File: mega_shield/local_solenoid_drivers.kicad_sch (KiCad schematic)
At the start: 15 parts, among them J21 1803277, J7 1803277, Q43 AO4486, Q44 AO4486, U29 NUP2202

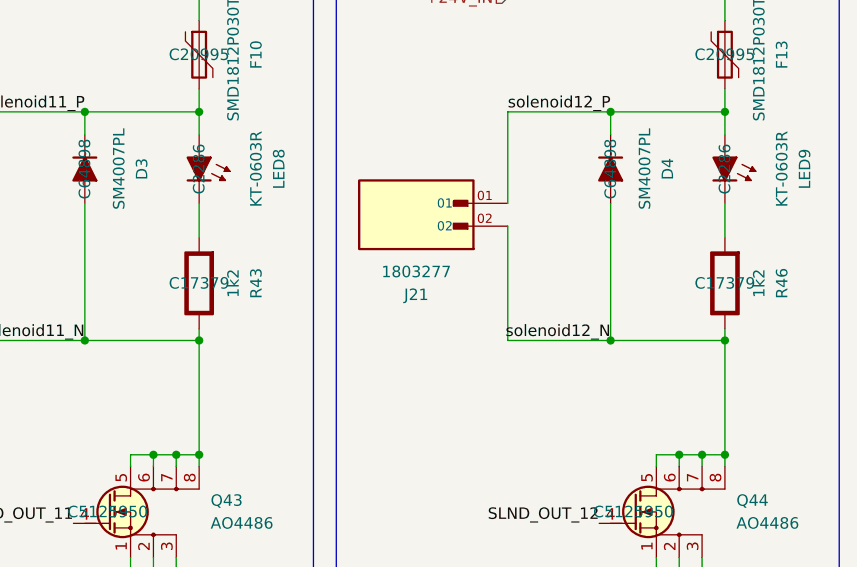
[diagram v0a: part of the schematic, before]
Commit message: updated jlcpcb number for the 1k2 resistors. Changed footprint from 0805 --> 0603.
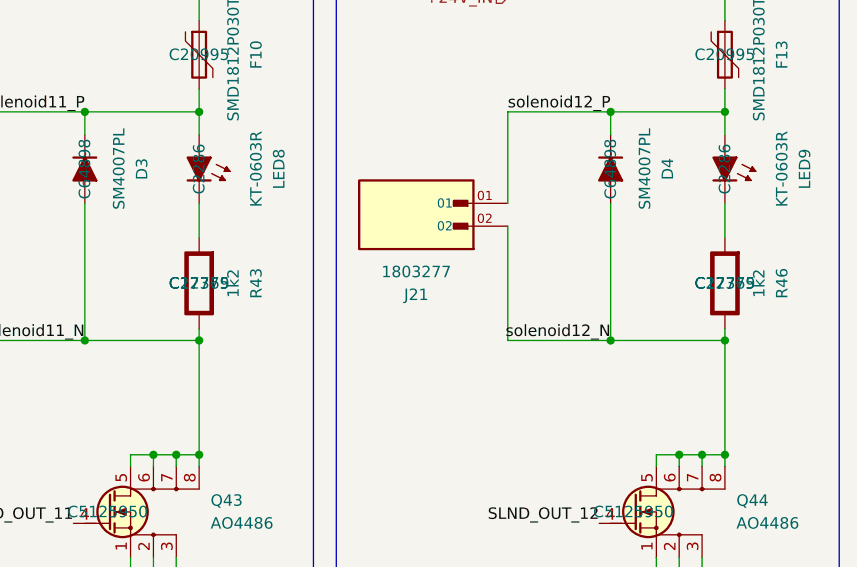
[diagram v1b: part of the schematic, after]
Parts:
- R43, R46: footprint Resistor_SMD:R_0805_2012Metric_Pad1.20x1.40mm_HandSolder -> Resistor_SMD:R_0201_0603Metric; jlcpcb (none) -> C22765
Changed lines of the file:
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@@
 			)
 		)
-		(property "Footprint" "Resistor_SMD:R_0805_2012Metric_Pad1.20x1.40mm_HandSolder"
+		(property "Footprint" "Resistor_SMD:R_0201_0603Metric"
 			(at 152.4 69.85 0)
 			(effects
@@
 		)
 		(property "JLCPCB" "C17379"
+			(at 152.4 69.85 0)
+			(effects
+				(font
+					(size 1.27 1.27)
+				)
+			)
+		)
+		(property "jlcpcb" "C22765"
 			(at 152.4 69.85 0)
 			(effects
@@
 			)
 		)
-		(property "Footprint" "Resistor_SMD:R_0805_2012Metric_Pad1.20x1.40mm_HandSolder"
+		(property "Footprint" "Resistor_SMD:R_0201_0603Metric"
 			(at 210.82 69.85 0)
 			(effects
@@
 			(at 210.82 69.85 0)
 			(effects
+				(font
+					(size 1.27 1.27)
+				)
+			)
+		)
+		(property "jlcpcb" "C22765"
+			(at 210.82 69.85 0)
+			(effects
